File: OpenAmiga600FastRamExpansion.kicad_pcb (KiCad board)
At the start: 2 copper layers, 71.8 x 72 mm, 11 parts, among them J1 MC68000_PLCC68, P1 JTAG_CONNECTOR, P99 OSHW_LOGO, U1 ATF1502AS-10JU44, U2 74LS157, U3 HYB5118160BSJ, U4 HYB5118160BSJ, U7 74LS157

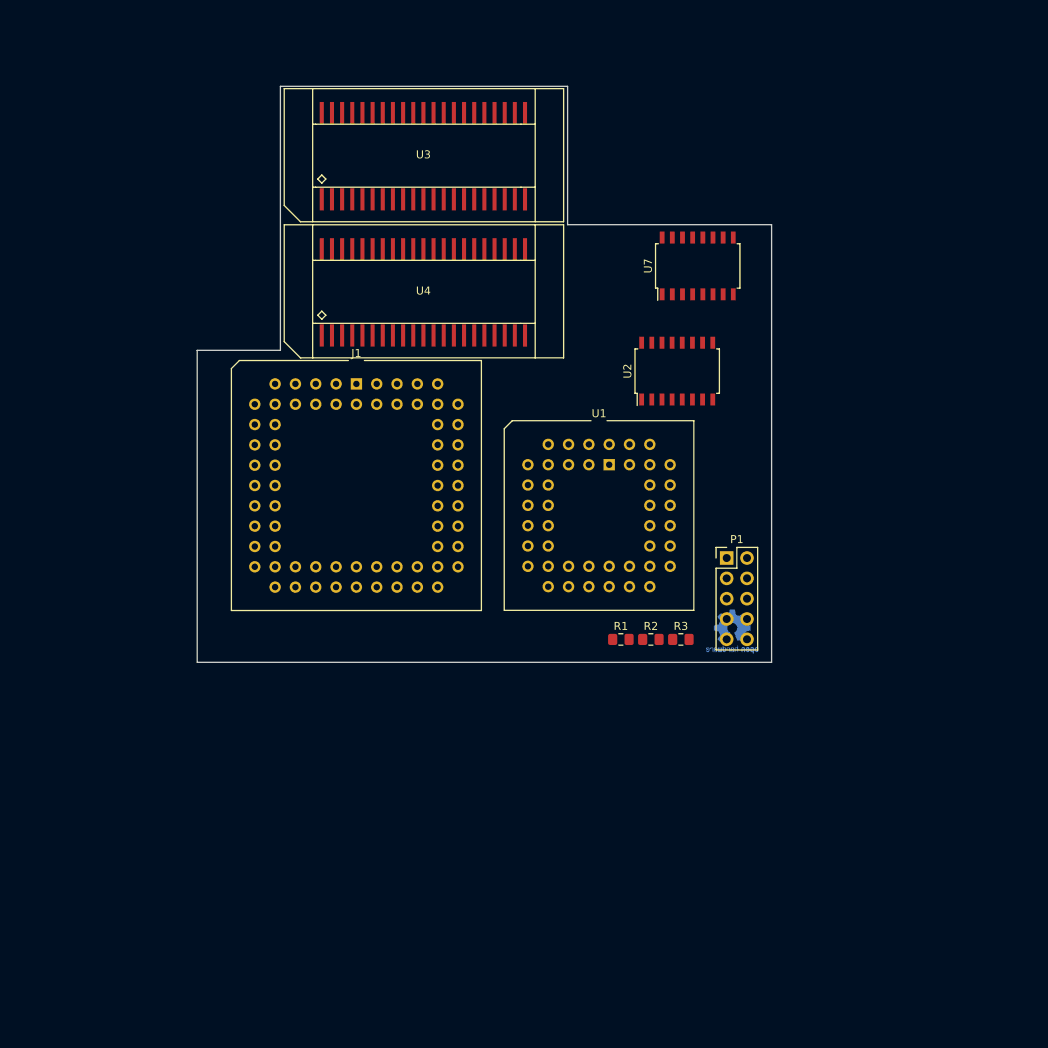
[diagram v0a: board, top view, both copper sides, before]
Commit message: Ready for routing!
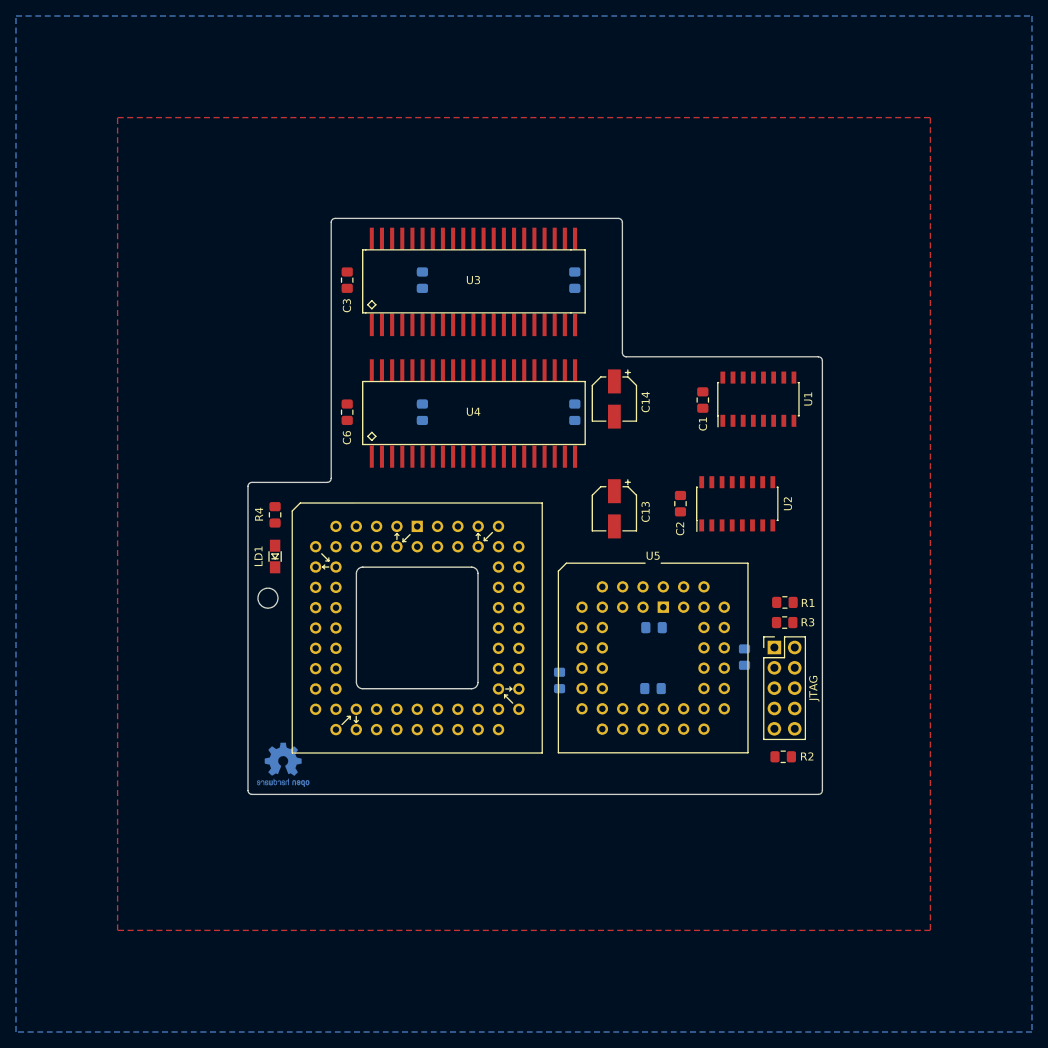
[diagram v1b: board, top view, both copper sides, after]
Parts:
- removed U7: 74LS157, Package_SO:SOIC-16W_5.3x10.2mm_P1.27mm
- added C1: 100n, Capacitor_SMD:C_0805_2012Metric_Pad1.15x1.40mm_HandSolder, F.Cu at (168.4, 77.2)
- added C10: 100n, Capacitor_SMD:C_0805_2012Metric_Pad1.15x1.40mm_HandSolder, B.Cu at (150.5, 112.3)
- added C11: 100n, Capacitor_SMD:C_0805_2012Metric_Pad1.15x1.40mm_HandSolder, B.Cu at (162.2, 113.3)
- added C12: 100n, Capacitor_SMD:C_0805_2012Metric_Pad1.15x1.40mm_HandSolder, B.Cu at (173.6, 109.3)
- added C13: 100n, Capacitor_SMD:CP_Elec_5x5.8, F.Cu at (157.3, 90.8)
- added C14: 100n, Capacitor_SMD:CP_Elec_5x5.8, F.Cu at (157.3, 77.1)
- added C2: 100n, Capacitor_SMD:C_0805_2012Metric_Pad1.15x1.40mm_HandSolder, F.Cu at (165.6, 90.2)
- added C3: 100n, Capacitor_SMD:C_0805_2012Metric_Pad1.15x1.40mm_HandSolder, F.Cu at (124.0, 62.2)
- added C4: 100n, Capacitor_SMD:C_0805_2012Metric_Pad1.15x1.40mm_HandSolder, B.Cu at (133.3, 62.2)
- added C5: 100n, Capacitor_SMD:C_0805_2012Metric_Pad1.15x1.40mm_HandSolder, B.Cu at (152.4, 62.2)
- added C6: 100n, Capacitor_SMD:C_0805_2012Metric_Pad1.15x1.40mm_HandSolder, F.Cu at (124.0, 78.7)
- added C7: 100n, Capacitor_SMD:C_0805_2012Metric_Pad1.15x1.40mm_HandSolder, B.Cu at (133.3, 78.7)
- added C8: 100n, Capacitor_SMD:C_0805_2012Metric_Pad1.15x1.40mm_HandSolder, B.Cu at (152.4, 78.7)
- added C9: 100n, Capacitor_SMD:C_0805_2012Metric_Pad1.15x1.40mm_HandSolder, B.Cu at (162.3, 105.7)
- added LD1: LED, OpenAmiga600FastRamExpansion:LED_0805_HandSoldering_ModSilkS, F.Cu at (114.9, 96.8)
- added P98: SCREW_HOLE, MountingHole:MountingHole_2.5mm, F.Cu at (114.0, 102.0)
- added R4: 10k, Resistor_SMD:R_0805_2012Metric_Pad1.15x1.40mm_HandSolder, F.Cu at (114.9, 91.6)
- added U5: ATF1502AS-10JU44, Package_LCC:PLCC-44_THT-Socket, F.Cu at (163.5, 103.1)
- J1: footprint Package_LCC:PLCC-68_THT-Socket -> OpenAmiga600FastRamExpansion:PLCC-68_THT-SocketUpsideDown
- U1: value ATF1502AS-10JU44 -> 74LS157; footprint Package_LCC:PLCC-44_THT-Socket -> Package_SO:SOIC-16_3.9x9.9mm_P1.27mm
- U2: footprint Package_SO:SOIC-16W_5.3x10.2mm_P1.27mm -> Package_SO:SOIC-16_3.9x9.9mm_P1.27mm
- U3, U4: footprint OpenAmiga600FastRamExpansion:SOJ-42-Socket-LongPads -> OpenAmiga600FastRamExpansion:SOJ-42-LongPads
- moved P99 58.5 mm to (116.0, 122.8)
- moved R2 22.1 mm to (178.4, 121.8)
- moved R1 21.0 mm to (178.7, 102.5), turned to 180 degrees
- moved U1 20.4 mm to (175.3, 77.1), turned to 90 degrees
- moved J1 19.4 mm to (132.7, 93.0)
- moved U2 18.2 mm to (172.7, 90.2)
- moved U3 16.9 mm to (139.7, 62.3)
- moved U4 16.4 mm to (139.7, 78.7)
- moved R3 13.1 mm to (178.6, 105.0), turned to 180 degrees
- moved P1 12.7 mm to (177.3, 108.2)
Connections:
- U1 pad 1: /~reset -> /mux_switch
- U1 pad 10: GND -> /a12
- U1 pad 11: /d15 -> /a9
- U1 pad 12: /a23 -> /ma9
- U1 pad 13: /jtag_tms -> /a11
- U1 pad 14: /a22 -> /a10
- U1 pad 15: VCC -> GND
- U1 pad 16: /a21 -> VCC
- U1 pad 2: /~as -> /a7
- U1 pad 3: VCC -> /a14
- U1 pad 4: /ma1 -> /ma6
- U1 pad 5: /ma0 -> /a8
- U1 pad 6: /d12 -> /a13
- U1 pad 7: /jtag_tdi -> /ma7
- U1 pad 8: /d13 -> GND
- U1 pad 9: /d14 -> /ma8
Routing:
- added copper zone on B.Cu, net GND
- added copper zone on F.Cu, net GND
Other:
- outline, holes or cut-outs redrawn
- net class Default: trace_width 0.25 -> 0.2; via_dia 0.8 -> 0.6
- net class Power added: clearance 0.2, trace_width 0.5, via_dia 0.8, via_drill 0.6
- board text added: "JTAG"
